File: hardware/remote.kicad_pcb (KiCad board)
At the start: 2 copper layers, 38.1 x 42.7 mm, 20 parts, among them SW1 SW_Push, SW2 SW_Push, SW3 SW_Push, SW4 SW_Push, SW5 SW_Push, SW6 SW_Push, U1 ATMEGA8-16AU

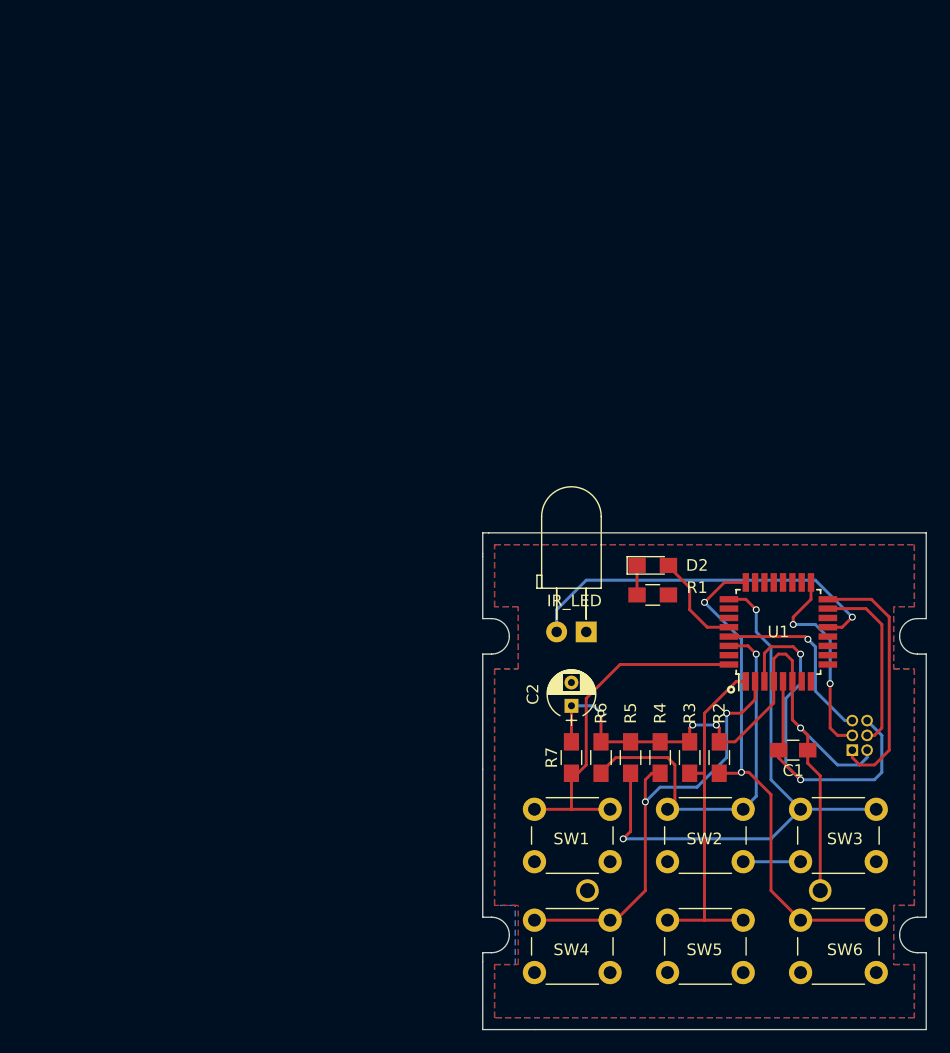
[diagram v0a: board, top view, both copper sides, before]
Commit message: Hardware update
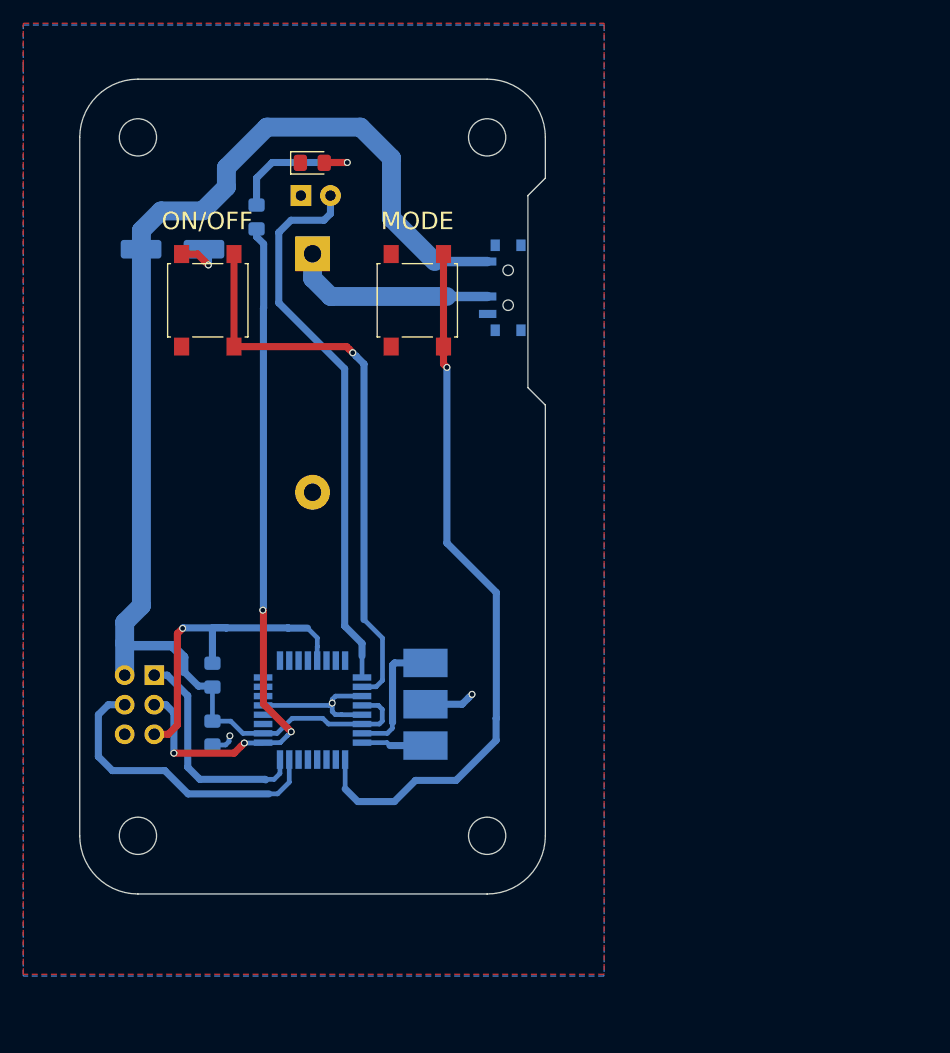
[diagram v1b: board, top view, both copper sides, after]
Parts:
- removed BATT1: CR2032, SF Batteries:BATTCOM_20MM_PTH
- removed ICSP: Conn_02x03_Odd_Even, Pin_Headers:Pin_Header_Straight_2x03_Pitch1.27mm
- removed IR_LED: IR_LED, LEDs:LED_D5.0mm_Horizontal_O3.81mm_Z3.0mm
- removed R3, R4, R5, R6, R7: 10K, Resistors_SMD:R_0805_HandSoldering
- removed SW2, SW3, SW4, SW5, SW6: SW_Push, Buttons_Switches_THT:SW_PUSH_6mm_h7.3mm
- added BT1: Battery_Cell, Battery:BatteryHolder_Keystone_107_1x23mm, B.Cu at (120.0, 38.0)
- added D1: LED, LED_THT:LED_D5.0mm_Horizontal_O1.27mm_Z3.0mm_IRBlack, B.Cu at (119.0, 33.0)
- added H1: MountingHole, MountingHole:MountingHole_3.2mm_M3, F.Cu at (105.0, 28.0)
- added H2: MountingHole, MountingHole:MountingHole_3.2mm_M3, F.Cu at (135.0, 28.0)
- added H3: MountingHole, MountingHole:MountingHole_3.2mm_M3, F.Cu at (135.0, 88.0)
- added H4: MountingHole, MountingHole:MountingHole_3.2mm_M3, F.Cu at (105.0, 88.0)
- added J1: AVR-ISP-6, Connector_PinHeader_2.54mm:PinHeader_2x03_P2.54mm_Vertical, B.Cu at (106.4, 74.2)
- added MODE: SW_Push, Button_Switch_SMD:SW_SPST_B3S-1000, F.Cu at (129.0, 42.0)
- added ON/OFF: SW_Push, Button_Switch_SMD:SW_SPST_B3S-1000, F.Cu at (111.0, 42.0)
- added Y1: Resonator_Small, Crystal:Resonator_SMD-3Pin_7.2x3.0mm_HandSoldering, B.Cu at (129.7, 76.7)
- C1: value 10nF -> C_Small; footprint Capacitors_SMD:C_0805_HandSoldering -> Capacitor_SMD:C_0805_2012Metric_Pad1.15x1.40mm_HandSolder; moved to B.Cu
- C2: value 10uF -> CP_Small; footprint Capacitors_THT:CP_Radial_D4.0mm_P2.00mm -> Capacitor_SMD:CP_Elec_6.3x4.5; moved to B.Cu
- D2: footprint LEDs:LED_0805_HandSoldering -> LED_SMD:LED_0805_2012Metric_Pad1.15x1.40mm_HandSolder
- R1: value 300 -> R_Small; footprint Resistors_SMD:R_0805_HandSoldering -> Resistor_SMD:R_0805_2012Metric_Pad1.15x1.40mm_HandSolder; moved to B.Cu
- R2: value 10K -> R_Small; footprint Resistors_SMD:R_0805_HandSoldering -> Resistor_SMD:R_0805_2012Metric_Pad1.15x1.40mm_HandSolder; moved to B.Cu
- SW1: value SW_Push -> SW_SPDT; footprint Buttons_Switches_THT:SW_PUSH_6mm_h7.3mm -> Button_Switch_SMD:SW_SPDT_PCM12; moved to B.Cu
- U1: value ATMEGA8-16AU -> ATMEGA328-AU; footprint Housings_QFP:TQFP-32_7x7mm_Pitch0.8mm -> Package_QFP:TQFP-32_7x7mm_P0.8mm; moved to B.Cu
- moved C2 52.1 mm to (108.0, 37.6), turned to 0 degrees
- moved C1 49.9 mm to (111.4, 79.2), turned to 270 degrees
- moved R1 47.0 mm to (115.2, 34.8), turned to 270 degrees
- moved D2 45.3 mm to (120.0, 30.2)
- moved SW1 44.9 mm to (136.5, 40.9), turned to 270 degrees
- moved R2 44.1 mm to (111.4, 74.2)
- moved U1 40.6 mm to (120.0, 77.2), turned to 180 degrees
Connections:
- C1 pad 1: +BATT -> VCC
- C2 pad 1: +BATT -> VCC
- D2 pad 1: Net-(D2-Pad1) -> GND
- R1 pad 1: GND -> Net-(D2-Pad2)
- R1 pad 2: Net-(D2-Pad1) -> LED_INFO
- R2 pad 1: BTN6 -> VCC
- R2 pad 2: +BATT -> RST
- SW1 pad 1: BTN1 -> VCC
- SW1 pad 2: GND -> Net-(BT1-Pad1)
- U1 pad 1: BTN5 -> LED_IR
- U1 pad 13: Net-(D1-Pad2) -> (no net)
- U1 pad 17: SCK -> LED_INFO
- U1 pad 18: (no net) -> VCC
- U1 pad 2: BTN4 -> BTN1
- U1 pad 21: (no net) -> GND
- U1 pad 24: BTN6 -> (no net)
- U1 pad 25: BTN3 -> (no net)
- U1 pad 28: Net-(D2-Pad2) -> (no net)
- U1 pad 29: RESET -> RST
- U1 pad 30: BTN2 -> (no net)
- U1 pad 32: BTN1 -> (no net)
- U1 pad 4: +BATT -> VCC
- U1 pad 6: +BATT -> VCC
- U1 pad 7: (no net) -> Net-(U1-Pad7)
- U1 pad 8: (no net) -> Net-(U1-Pad8)
- U1 pad 9: (no net) -> BTN2
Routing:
- net VCC: track 0.00 -> 112.5 mm
- net +BATT: track 62.2 -> 0.00 mm, vias 4 -> 0
- net LED_INFO: track 0.00 -> 60.8 mm, vias 0 -> 5
- net BTN3: track 50.1 -> 0.00 mm, vias 2 -> 0
- net LED_IR: track 0.00 -> 47.9 mm
- net BTN6: track 44.0 -> 0.00 mm, vias 2 -> 0
- net BTN4: track 39.1 -> 0.00 mm, vias 2 -> 0
- net Net-(D1-Pad2): track 32.1 -> 0.00 mm, vias 1 -> 0
- net BTN5: track 32.0 -> 0.00 mm
- net RST: track 0.00 -> 29.0 mm, vias 0 -> 1
- net BTN2: track 34.9 -> 61.8 mm
- net GND: track 44.4 -> 22.5 mm, vias 2 -> 4
- net BTN1: track 30.3 -> 49.6 mm, vias 0 -> 1
- net Net-(BT1-Pad1): track 0.00 -> 17.8 mm
- net SCK: track 17.7 -> 0.00 mm, vias 2 -> 0
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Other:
- board size 38.1 x 42.7 mm -> 40 x 70 mm
- board text added: "CR2032 - 3V"
- board text added: "Rev 1.0 - Feb 2021"
- board text added: "Whisperpool Remote"
- board text removed: "Whirlpool remote Rev 1"
